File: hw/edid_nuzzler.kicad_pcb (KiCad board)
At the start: 4 copper layers, 49 x 32 mm, 42 parts, among them J1 HDMI_A, J2 HDMI_A, J3 Conn_02x03_Counter_Clockwise, J4 USB_C_Receptacle_USB2.0_16P, Q1 BSS84AK, SW1 SW_Push, U1 74LVC1G3157, U2 74LVC1G3157, U3 CH340N, U4 CH32V003AxMx, U5 74LVC1G3157

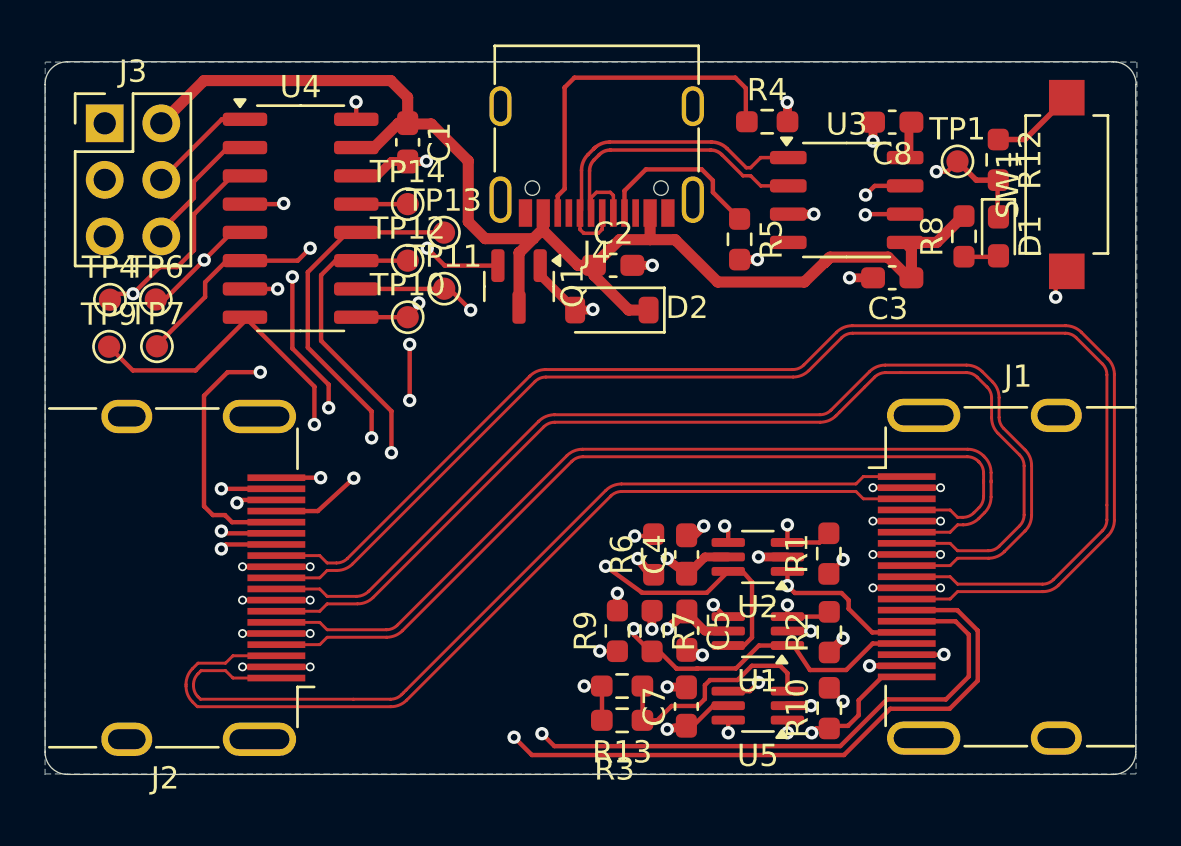
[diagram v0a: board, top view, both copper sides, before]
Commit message: Mostly done
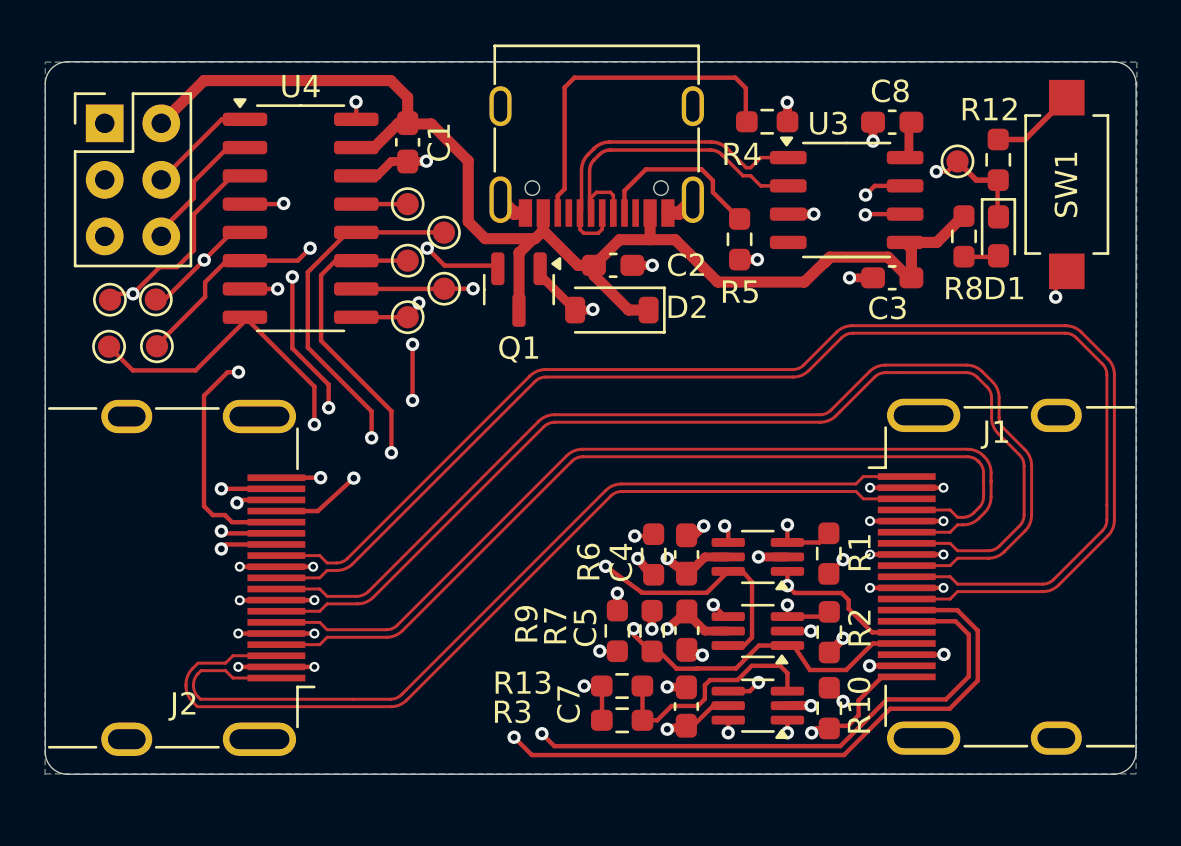
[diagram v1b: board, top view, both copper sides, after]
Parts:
- moved Q1 0.14 mm to (182.7, 72.3)
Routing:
- net GND: track 44.0 -> 48.8 mm
- net Net-(U3-TXD): track 26.8 -> 26.0 mm
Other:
- board text added: "Camp++"
- board text added: "Notices EDID OwO whats this?"
